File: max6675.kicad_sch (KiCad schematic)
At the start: 8 parts, among them J12 Conn_01x02_Socket, U12 MAX6675ISA+T, U7 MAX31855KASA

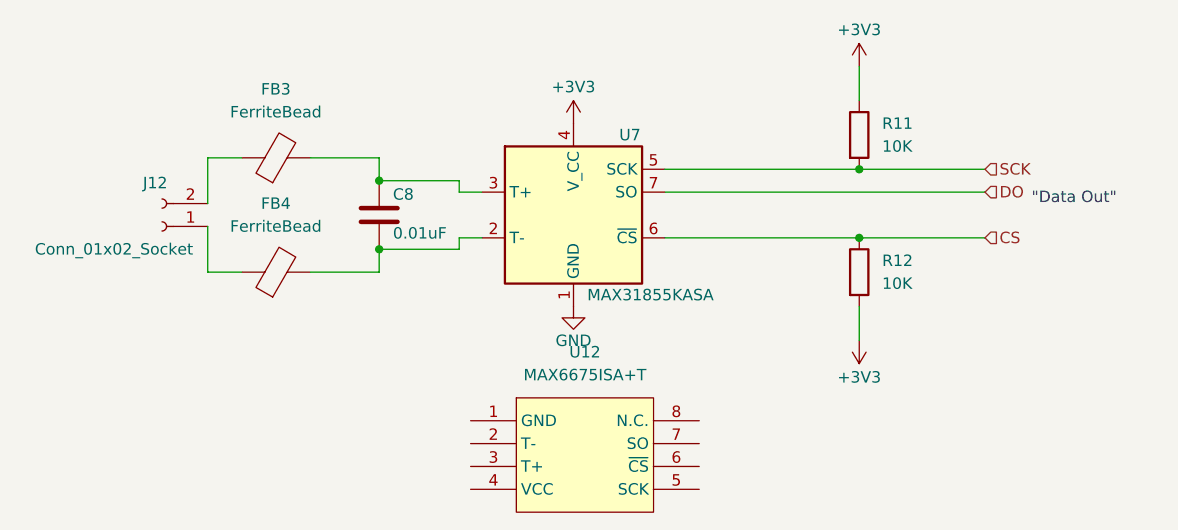
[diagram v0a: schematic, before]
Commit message: almost there
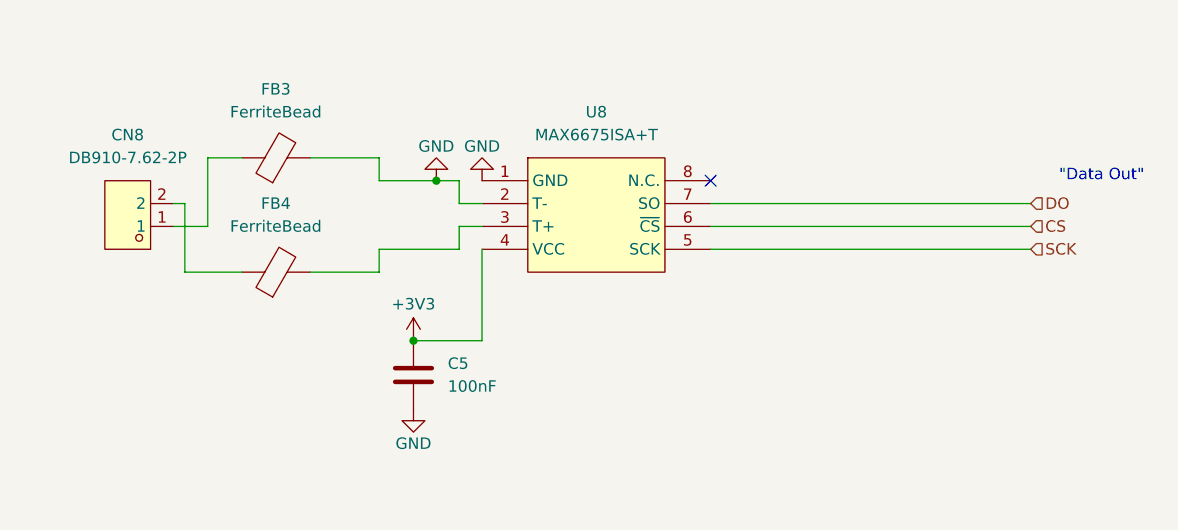
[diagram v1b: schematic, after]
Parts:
- removed C8: 0.01uF, Capacitor_SMD:C_0402_1005Metric, symbol Device:C
- removed J12: Conn_01x02_Socket, TerminalBlock:TerminalBlock_bornier-2_P5.08mm, symbol Connector:Conn_01x02_Socket
- removed R11, R12: 10K, Resistor_SMD:R_0603_1608Metric, symbol Device:R
- removed U7: MAX31855KASA, Package_SO:SOIC-8_3.9x4.9mm_P1.27mm, symbol Sensor_Temperature:MAX31855KASA
- added C5: 100nF, Capacitor_SMD:C_0402_1005Metric, symbol Device:C
- added CN8: DB910-7.62-2P, blastLib:CONN-TH_2P-P7.62_DB910-7.62-2P, symbol blastLib:DB910-7.62-2P
- renumbered U12 to U8
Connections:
- net +3V3: now also U8.4 (VCC), C5.1
- net CS: now also U8.6 (~{CS})
- net DO: now also U8.7 (SO)
- net GND: now also FB3.2, U8.1 (GND), U8.2 (T-), C5.2
- net SCK: now also U8.5 (SCK)
- net at FB4.1: now also CN8.2
- net at FB4.2: now also U8.3 (T+)
- net at FB3.1: now also CN8.1
- no-connect marks 0 -> 1
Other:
- moved on the sheet: U8
